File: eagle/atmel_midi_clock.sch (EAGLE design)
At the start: 46 parts, among them IC1 TL084P, IC2 40106N, U1 ATMEGA328P_PDIP, X1 22-23-2031, X2 22-23-2031, X3 22-23-2031, X4 22-23-2031

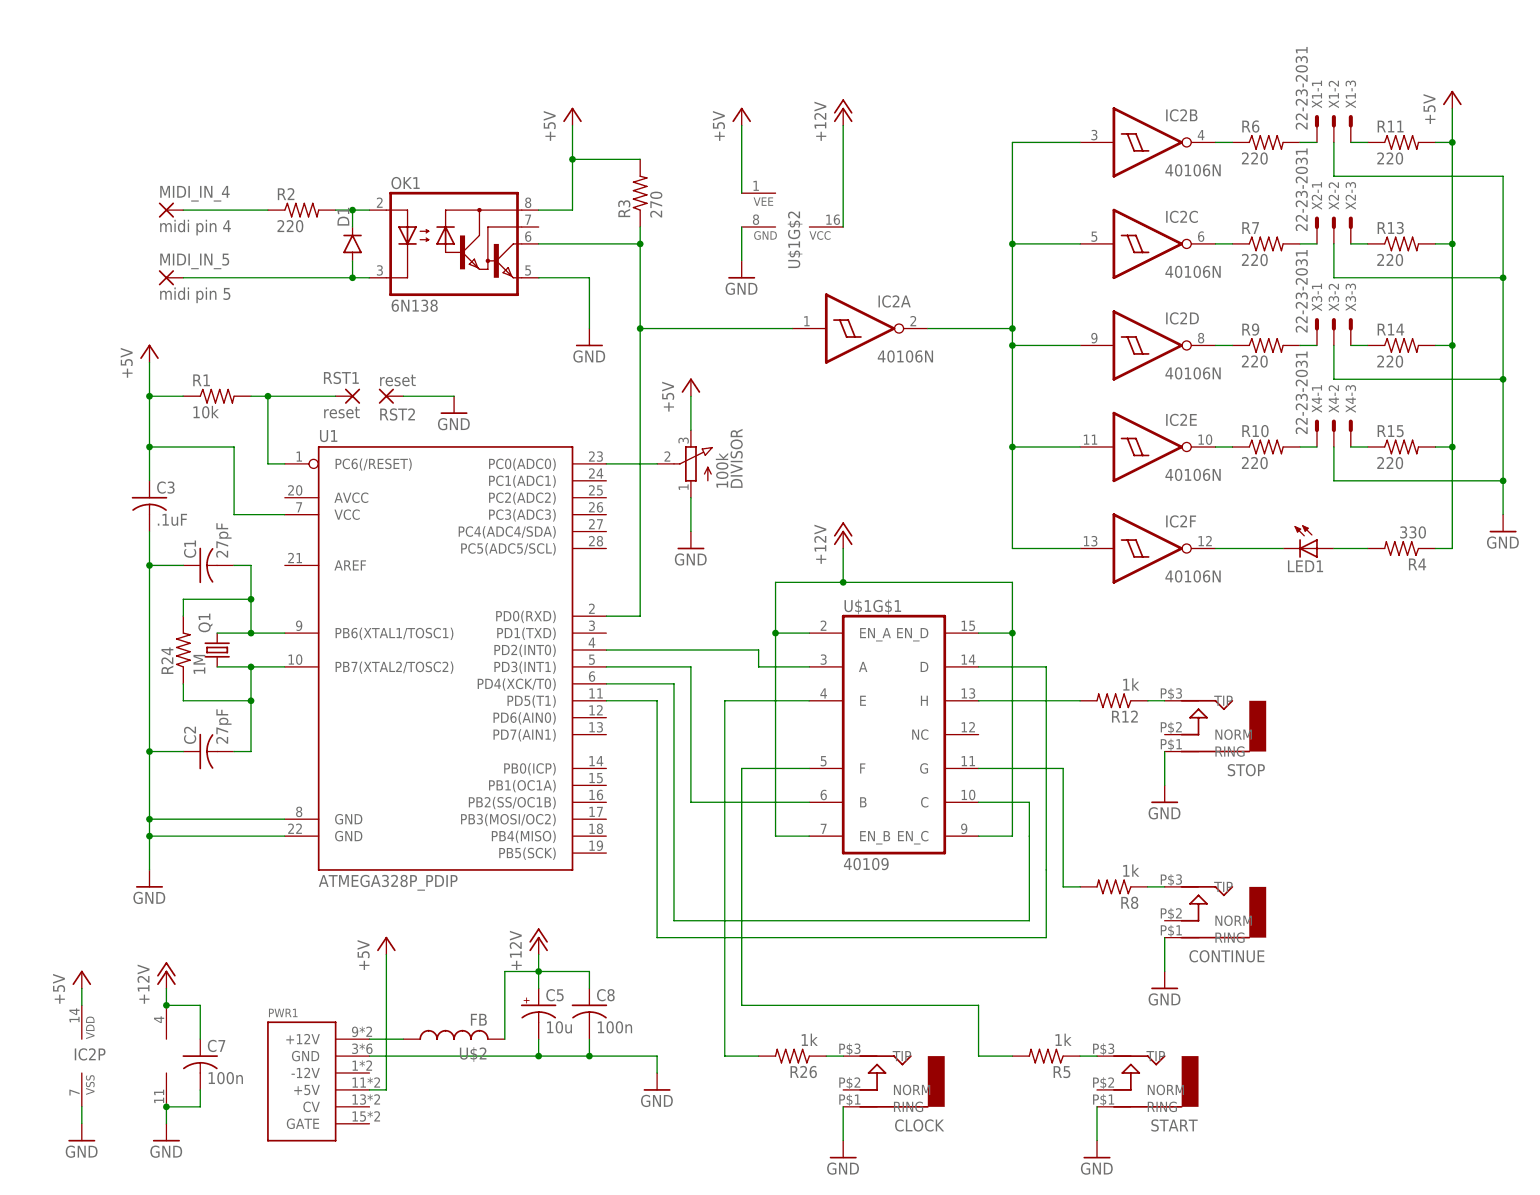
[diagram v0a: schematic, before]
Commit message: midi thrus and leds
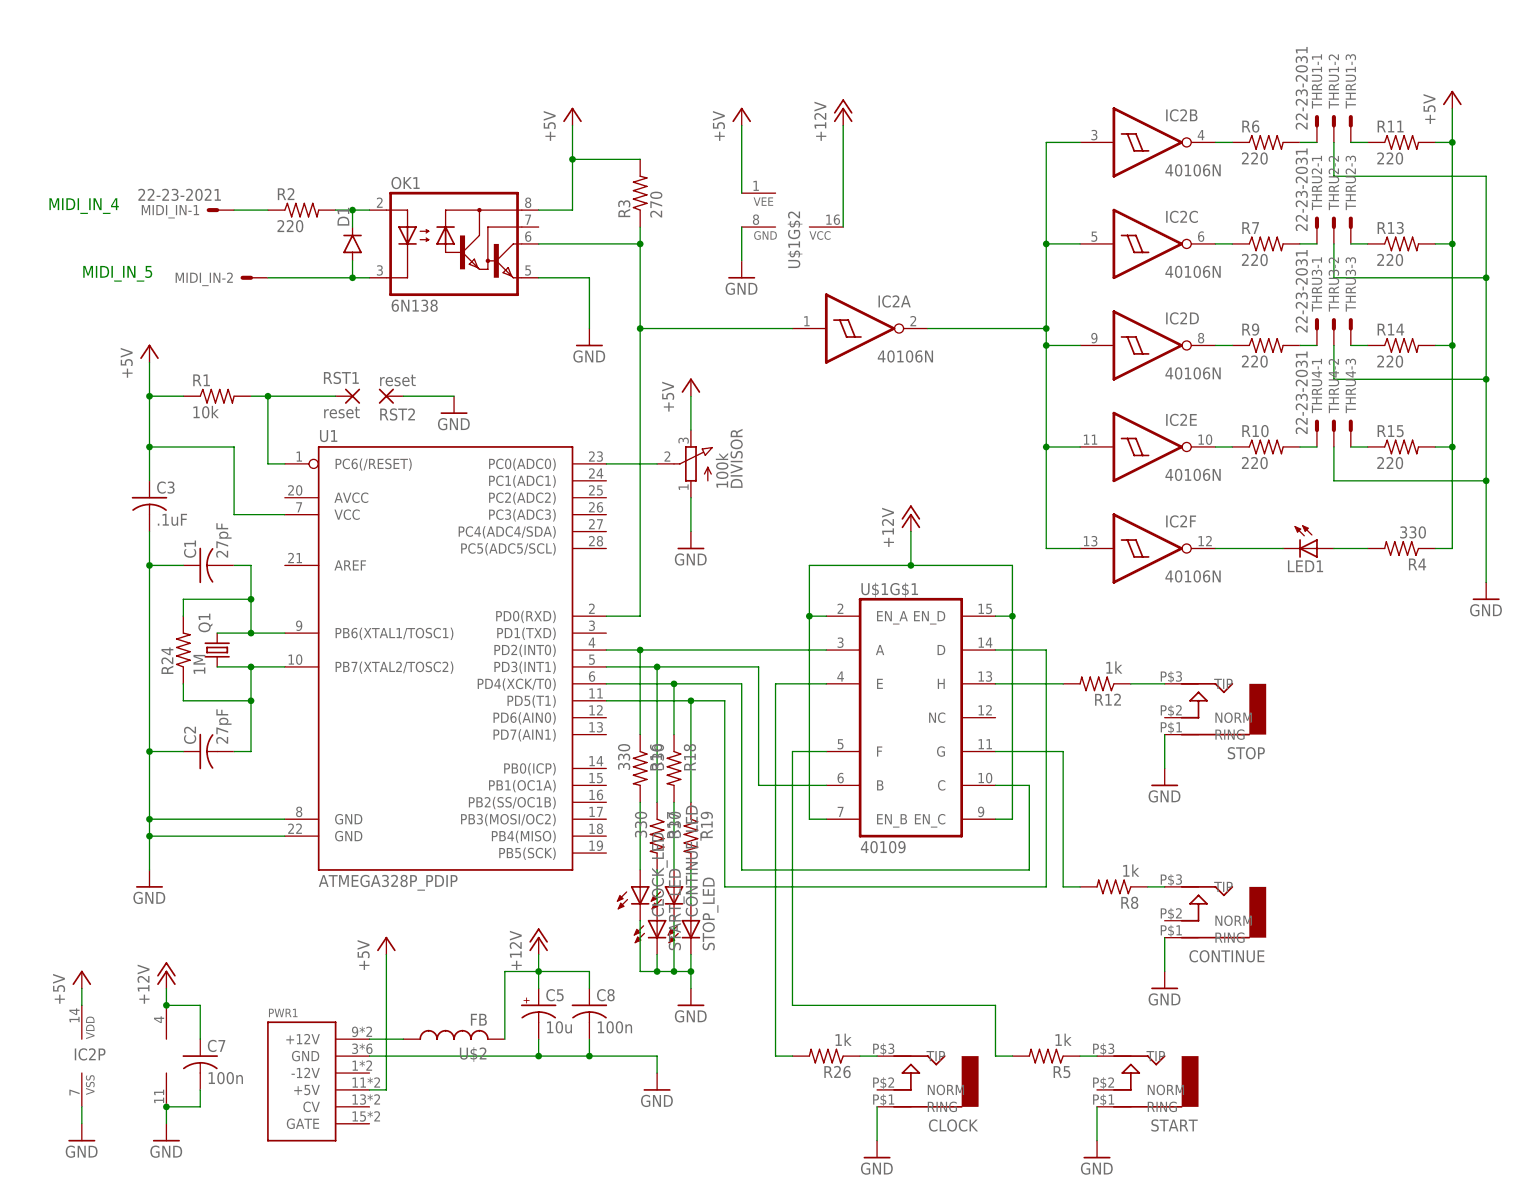
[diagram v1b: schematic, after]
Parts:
- removed MIDI_IN_4: midi pin 4, wirepad:2,54/0,9
- removed MIDI_IN_5: midi pin 5, wirepad:2,54/0,9
- added CLOCK_LED, CONTINUE_LED, START_LED, STOP_LED: (no value), led:LED5MM
- added MIDI_IN: 22-23-2021, con-molex:22-23-2021
- added R16, R17, R18, R19: 330, rcl:R-US_0207/10
- renumbered X1 to THRU1, X2 to THRU2, X3 to THRU3, X4 to THRU4
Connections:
- new net N$37: R17.2, START_LED.A
- new net N$38: CLOCK_LED.A, R16.2
- new net N$39: CONTINUE_LED.A, R18.2
- new net N$40: R19.2, STOP_LED.A
- net GND: now also CLOCK_LED.C, CONTINUE_LED.C, START_LED.C, STOP_LED.C
- net N$1: now also R18.1
- net N$10: now also R17.1
- net N$3: now also MIDI_IN-2.S; no longer MIDI_IN_5.P
- net N$6: now also R19.1
- net N$8: now also MIDI_IN-1.S; no longer MIDI_IN_4.P
- net N$9: now also R16.1
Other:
- note added: "MIDI_IN_4"
- note added: "MIDI_IN_5"
- moved on the sheet: CLOCK, R12, R26, STOP, U$1G$1

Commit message: layout begins
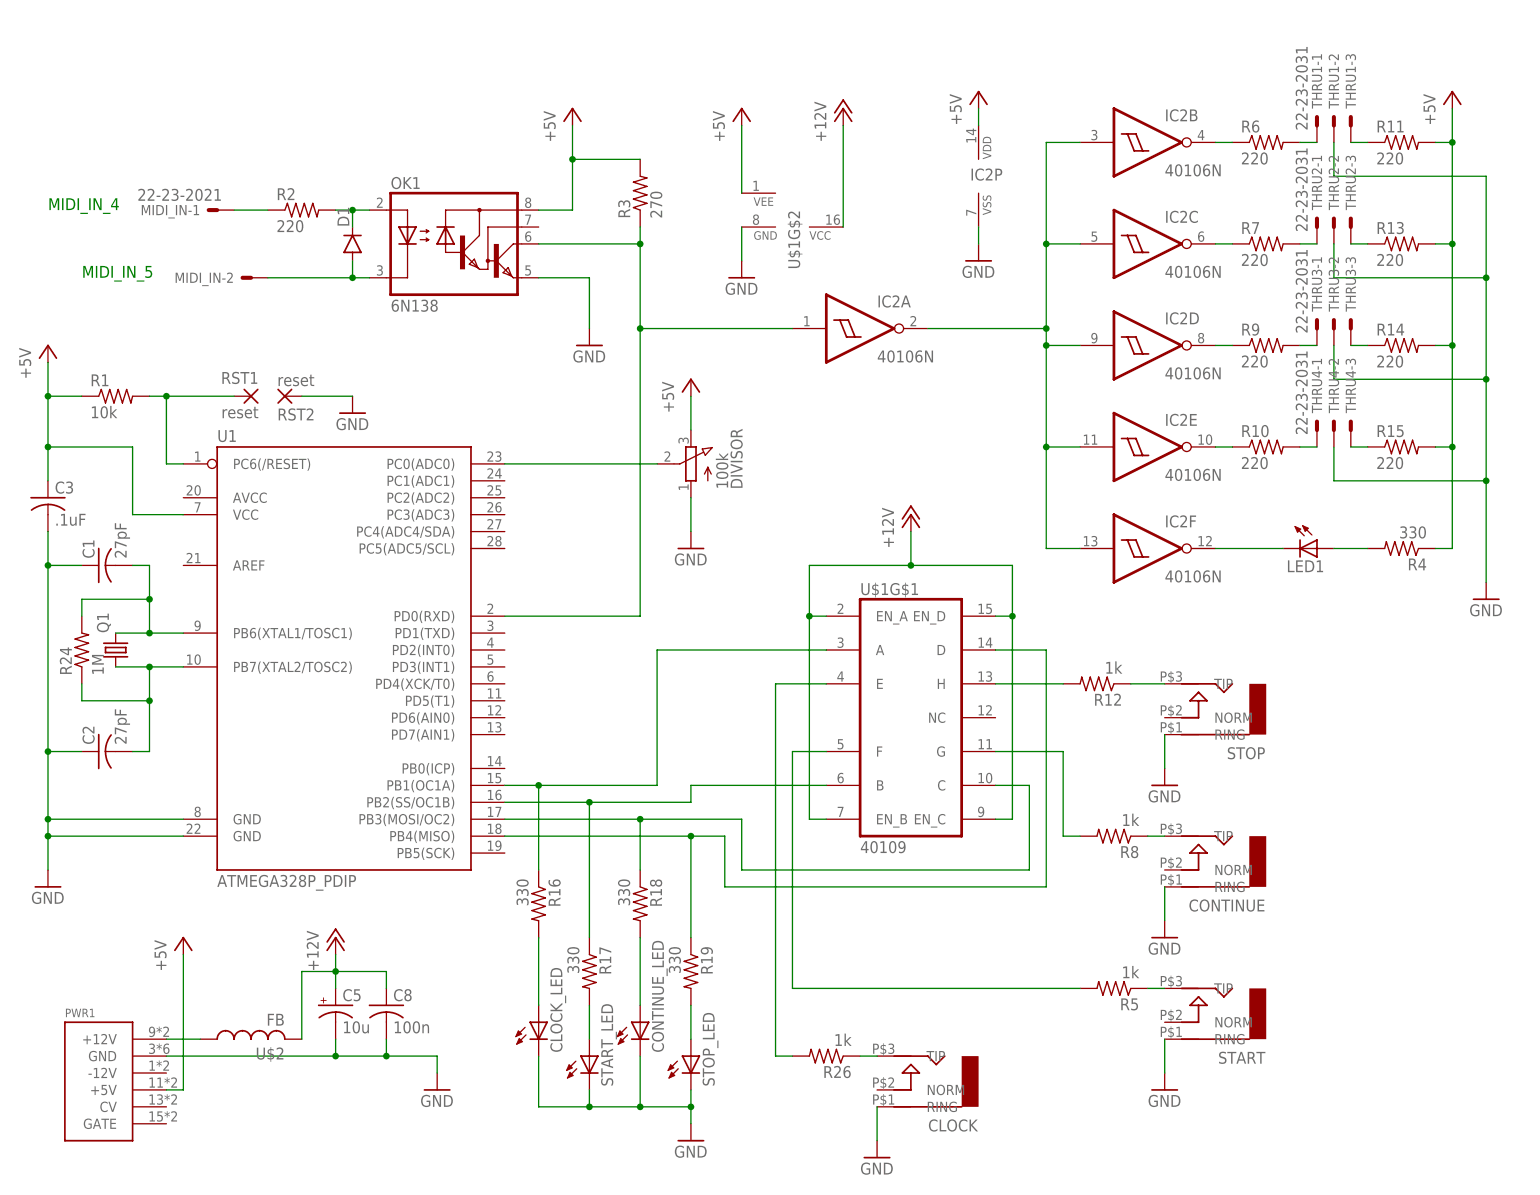
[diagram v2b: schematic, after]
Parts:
- removed C7: 100n, rcl:C-US050-024X044
- removed IC1: TL084P, linear:TL084P
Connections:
- net +12V: no longer C7.1, IC1P.V+
- net N$1: now also U1.PB3(MOSI/OC2); no longer U1.PD4(XCK/T0)
- net N$10: now also U1.PB2(SS/OC1B); no longer U1.PD3(INT1)
- net N$29: no longer C7.2, IC1P.V-
- net N$6: now also U1.PB4(MISO); no longer U1.PD5(T1)
- net N$9: now also U1.PB1(OC1A); no longer U1.PD2(INT0)
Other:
- moved on the sheet: C1, C2, C3, C5, C8, CLOCK_LED, CONTINUE, CONTINUE_LED, IC2P, PWR1, Q1, R1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
